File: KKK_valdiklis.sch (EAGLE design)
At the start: 62 parts, among them IC2 L293D, IC4 ATMEGA1284, IC5 DS1307, J4 HEAD3X2, K1 S202T02, K2 S202T02, K3 S202T02, K4 S202T02, K5 S202T02, K6 S202T02, Q2 TIP120V, Q4 32.768, X1 Boiler pump, X10 22-23-2031, X11 +12V, X2 Storage tank pump, X3 Radiator pump, X4 4 way valve 1, X5 4 way valve 2, X6 Floor heating, X7 motorized valve 1, X77 PUMP1, X8 motorized valve 2, X9 16MHz

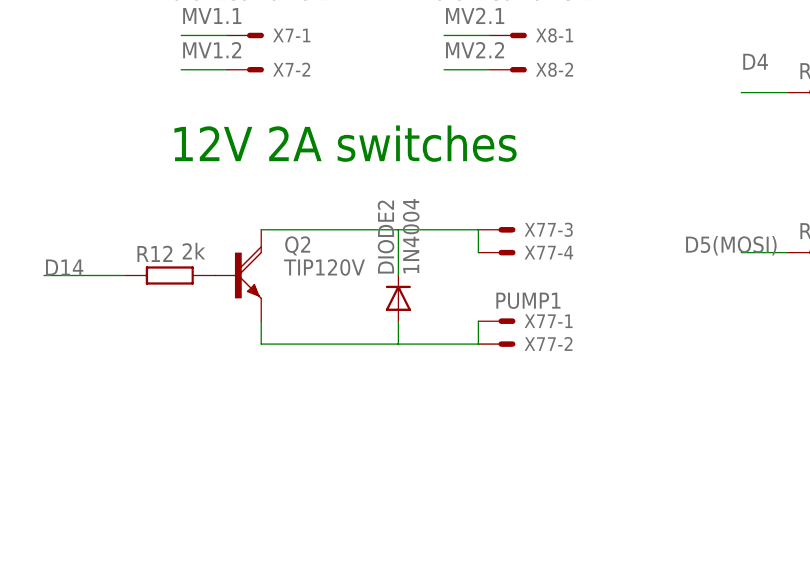
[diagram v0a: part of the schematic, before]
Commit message: trasavimas
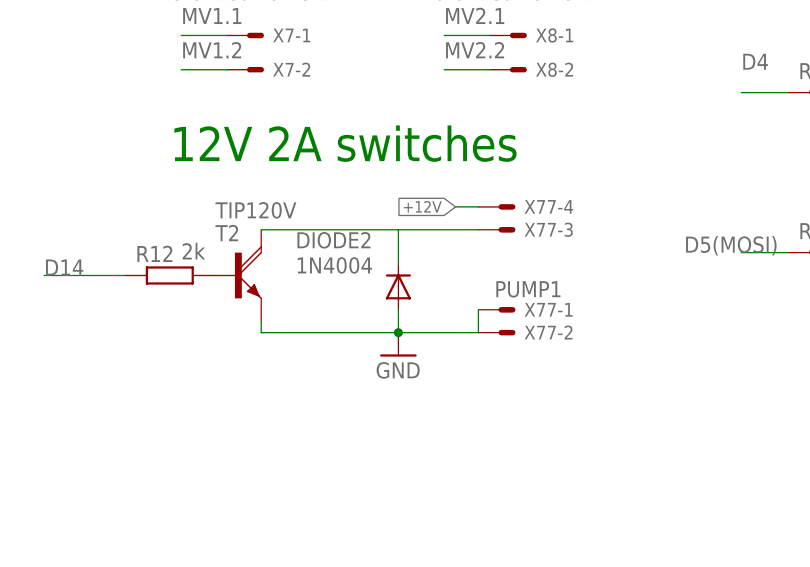
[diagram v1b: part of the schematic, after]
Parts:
- renumbered Q2 to T2
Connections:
- removed net N$5: IC2.VCC2, X11-2.S
- new net +12V: IC2.VCC2, X11-2.S, X77-4.S
- net N$15: no longer X77-4.S
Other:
- moved on the sheet: DIODE2, X77-1, X77-2, X77-4
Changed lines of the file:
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@@
 <part name="R9" library="resistor" deviceset="R-EU_" device="0207/10" value="1k"/>
 <part name="R11" library="resistor" deviceset="R-EU_" device="0207/10" value="2k"/>
-<part name="Q2" library="rocketfarm" deviceset="TIP120" device="V"/>
+<part name="T2" library="rocketfarm" deviceset="TIP120" device="V"/>
 <part name="X77" library="con-molex" deviceset="22-23-2041" device="" value="PUMP1"/>
 <part name="R12" library="resistor" deviceset="R-EU_" device="0207/10" value="2k"/>
@@
 <part name="X11" library="con-molex" deviceset="22-23-2021" device="" value="+12V"/>
 <part name="GND14" library="SparkFun-Aesthetics" deviceset="GND" device=""/>
+<part name="GND19" library="SparkFun-Aesthetics" deviceset="GND" device=""/>
 </parts>
 <sheets>
@@
 <instance part="R9" gate="G$1" x="175.26" y="7.62" rot="R90"/>
 <instance part="R11" gate="G$1" x="175.26" y="22.86" rot="R90"/>
-<instance part="Q2" gate="1" x="-76.2" y="76.2"/>
-<instance part="X77" gate="-1" x="-46.99" y="71.12"/>
-<instance part="X77" gate="-2" x="-46.99" y="68.58"/>
+<instance part="T2" gate="1" x="-76.2" y="76.2" smashed="yes">
+<attribute name="NAME" x="-78.74" y="80.01" size="1.778" layer="95"/>
+<attribute name="VALUE" x="-78.74" y="82.55" size="1.778" layer="96"/>
+</instance>
+<instance part="X77" gate="-1" x="-46.99" y="72.39"/>
+<instance part="X77" gate="-2" x="-46.99" y="69.85"/>
 <instance part="X77" gate="-3" x="-46.99" y="81.28"/>
-<instance part="X77" gate="-4" x="-46.99" y="78.74"/>
+<instance part="X77" gate="-4" x="-46.99" y="83.82"/>
 <instance part="R12" gate="G$1" x="-83.82" y="76.2" smashed="yes">
 <attribute name="NAME" x="-87.63" y="77.6986" size="1.778" layer="95"/>
 <attribute name="VALUE" x="-82.55" y="77.978" size="1.778" layer="96"/>
 </instance>
-<instance part="DIODE2" gate="1" x="-58.42" y="73.66" rot="R90"/>
+<instance part="DIODE2" gate="1" x="-58.42" y="74.93" smashed="yes" rot="R90">
+<attribute name="NAME" x="-69.85" y="79.2226" size="1.778" layer="95"/>
+<attribute name="VALUE" x="-69.85" y="76.4286" size="1.778" layer="96"/>
+</instance>
 <instance part="Q4" gate="G$1" x="142.24" y="91.44" rot="R180"/>
 <instance part="IC5" gate="G$1" x="144.78" y="68.58"/>
@@
 <instance part="X11" gate="-2" x="-86.36" y="119.38" rot="R180"/>
 <instance part="GND14" gate="1" x="-77.47" y="114.3"/>
+<instance part="GND19" gate="1" x="-58.42" y="67.31"/>
 </instances>
 <busses>
@@
 </segment>
 <segment>
-<pinref part="Q2" gate="1" pin="E"/>
-<wire x1="-73.66" y1="71.12" x2="-73.66" y2="68.58" width="0.1524" layer="91"/>
-<wire x1="-73.66" y1="68.58" x2="-58.42" y2="68.58" width="0.1524" layer="91"/>
+<pinref part="T2" gate="1" pin="E"/>
+<wire x1="-73.66" y1="71.12" x2="-73.66" y2="69.85" width="0.1524" layer="91"/>
+<wire x1="-73.66" y1="69.85" x2="-58.42" y2="69.85" width="0.1524" layer="91"/>
 <pinref part="DIODE2" gate="1" pin="A"/>
-<wire x1="-58.42" y1="71.12" x2="-58.42" y2="68.58" width="0.1524" layer="91"/>
-<wire x1="-58.42" y1="68.58" x2="-49.53" y2="68.58" width="0.1524" layer="91"/>
+<wire x1="-58.42" y1="72.39" x2="-58.42" y2="69.85" width="0.1524" layer="91"/>
+<wire x1="-58.42" y1="69.85" x2="-49.53" y2="69.85" width="0.1524" layer="91"/>
 <pinref part="X77" gate="-2" pin="S"/>
 <pinref part="X77" gate="-1" pin="S"/>
-<wire x1="-49.53" y1="68.58" x2="-49.53" y2="71.12" width="0.1524" layer="91"/>
+<wire x1="-49.53" y1="69.85" x2="-49.53" y2="72.39" width="0.1524" layer="91"/>
+<pinref part="GND19" gate="1" pin="GND"/>
+<junction x="-58.42" y="69.85"/>
 </segment>
 <segment>
@@
 <segment>
 <pinref part="R12" gate="G$1" pin="2"/>
-<pinref part="Q2" gate="1" pin="B"/>
+<pinref part="T2" gate="1" pin="B"/>
 </segment>
 </net>
 <net name="N$15" class="0">
 <segment>
-<pinref part="Q2" gate="1" pin="C"/>
+<pinref part="T2" gate="1" pin="C"/>
 <wire x1="-73.66" y1="81.28" x2="-58.42" y2="81.28" width="0.1524" layer="91"/>
 <wire x1="-58.42" y1="81.28" x2="-49.53" y2="81.28" width="0.1524" layer="91"/>
 <pinref part="DIODE2" gate="1" pin="C"/>
-<wire x1="-58.42" y1="76.2" x2="-58.42" y2="81.28" width="0.1524" layer="91"/>
+<wire x1="-58.42" y1="77.47" x2="-58.42" y2="81.28" width="0.1524" layer="91"/>
 <pinref part="X77" gate="-3" pin="S"/>
-<pinref part="X77" gate="-4" pin="S"/>
-<wire x1="-49.53" y1="81.28" x2="-49.53" y2="78.74" width="0.1524" layer="91"/>
 </segment>
 </net>
@@
 </segment>
 </net>
-<net name="N$5" class="0">
+<net name="+12V" class="0">
+<segment>
+<pinref part="X77" gate="-4" pin="S"/>
+<wire x1="-49.53" y1="83.82" x2="-52.07" y2="83.82" width="0.2032" layer="91"/>
+<label x="-52.07" y="83.82" size="1.27" layer="95" rot="R180" xref="yes"/>
+</segment>
 <segment>
 <pinref part="IC2" gate="G$1" pin="VCC2"/>
